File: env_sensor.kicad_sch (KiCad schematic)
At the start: 40 parts, among them J1 E Paper, J10 PWMOUT, J15 MH-Z19, J16 ADCs, J18 Conn_01x02_Pin, J3 Barrel_Jack, J4 LED_OUTPUT, J7 USB_C_Receptacle_USB2.0_16P, J8 v5_v3, J9 DEBUG, Q1 NMOS, Q2 NMOS, Q3 NMOS, SW1 EN, SW2 BOOT, U3 ESP32-S3-WROOM-1, U4 TXB0104PW, U6 TPS2065CDBV, U7 AP7361C-33E, Y1 Crystal

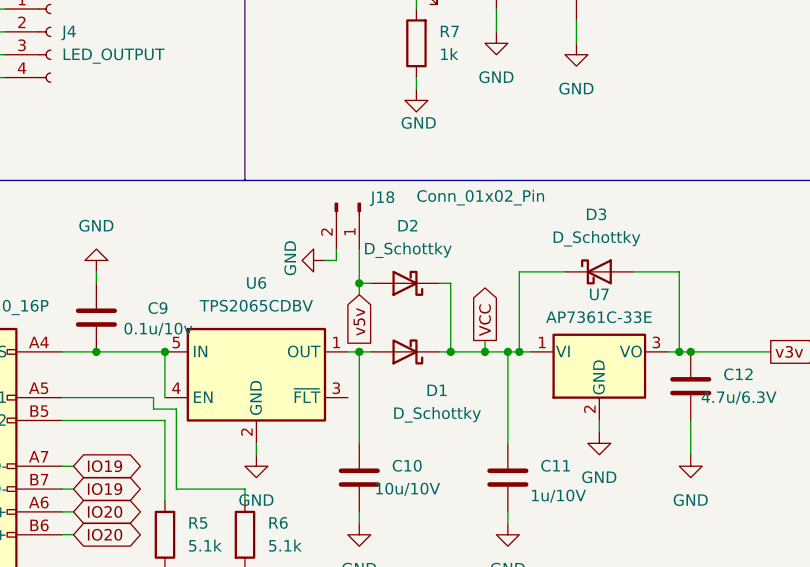
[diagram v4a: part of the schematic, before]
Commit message: update BOM
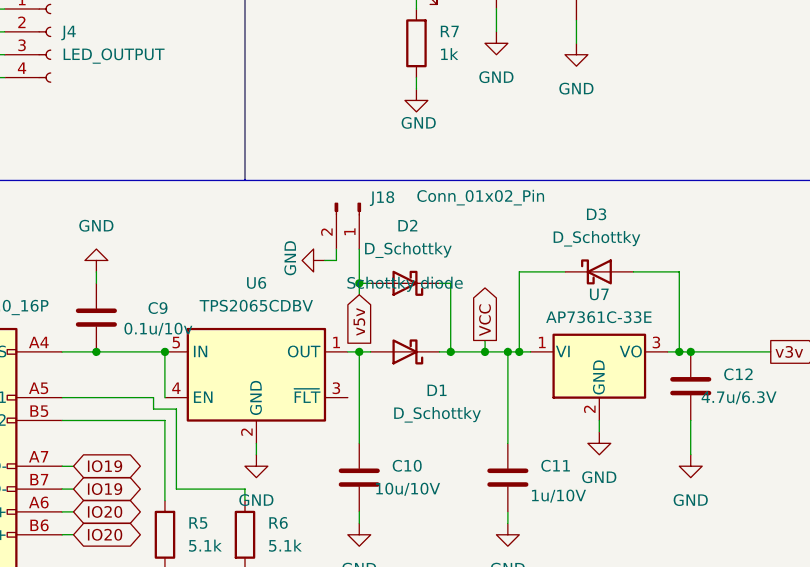
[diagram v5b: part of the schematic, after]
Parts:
- C7, C9: LCSC (none) -> C1853272
- D1, D2, D3: LCSC C86598 -> C123070
- R4: LCSC (none) -> C25804
- R5, R6: LCSC (none) -> C23186
- U6: LCSC (none) -> C353882
- U7: LCSC (none) -> C500795
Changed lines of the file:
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@@
 			)
 		)
-		(property "LCSC" ""
+		(property "LCSC" "C1853272"
 			(at 53.34 148.59 90)
 			(effects
@@
 			)
 		)
-		(property "LCSC" ""
+		(property "LCSC" "C25804"
 			(at 144.78 41.91 0)
 			(effects
@@
 			)
 		)
+		(property "LCSC" "C500795"
+			(at 109.22 152.4 0)
+			(effects
+				(font
+					(size 1.27 1.27)
+				)
+				(hide yes)
+			)
+		)
 		(pin "1"
 		)
@@
 			)
 		)
-		(property "LCSC" ""
+		(property "LCSC" "C23186"
 			(at 60.96 172.72 0)
 			(effects
@@
 			)
 		)
-		(property "LCSC" "C86598"
+		(property "LCSC" "C123070"
 			(at 109.22 143.51 0)
 			(effects
@@
 			)
 		)
-		(property "LCSC" ""
+		(property "LCSC" "C1853272"
 			(at 175.26 41.91 90)
 			(effects
@@
 			)
 		)
+		(property "LCSC" "C353882"
+			(at 71.12 154.94 0)
+			(effects
+				(font
+					(size 1.27 1.27)
+				)
+				(hide yes)
+			)
+		)
 		(pin "1"
 		)
@@
 			)
 		)
-		(property "LCSC" "C86598"
+		(property "LCSC" "C123070"
 			(at 87.63 152.4 0)
 			(effects
@@
 			)
 		)
-		(property "LCSC" ""
+		(property "LCSC" "C23186"
 			(at 69.85 172.72 0)
 			(effects
@@
 					(size 1.27 1.27)
 				)
-				(hide yes)
 			)
 		)
-		(property "LCSC" "C86598"
+		(property "LCSC" "C123070"
 			(at 87.63 144.78 0)
 			(effects

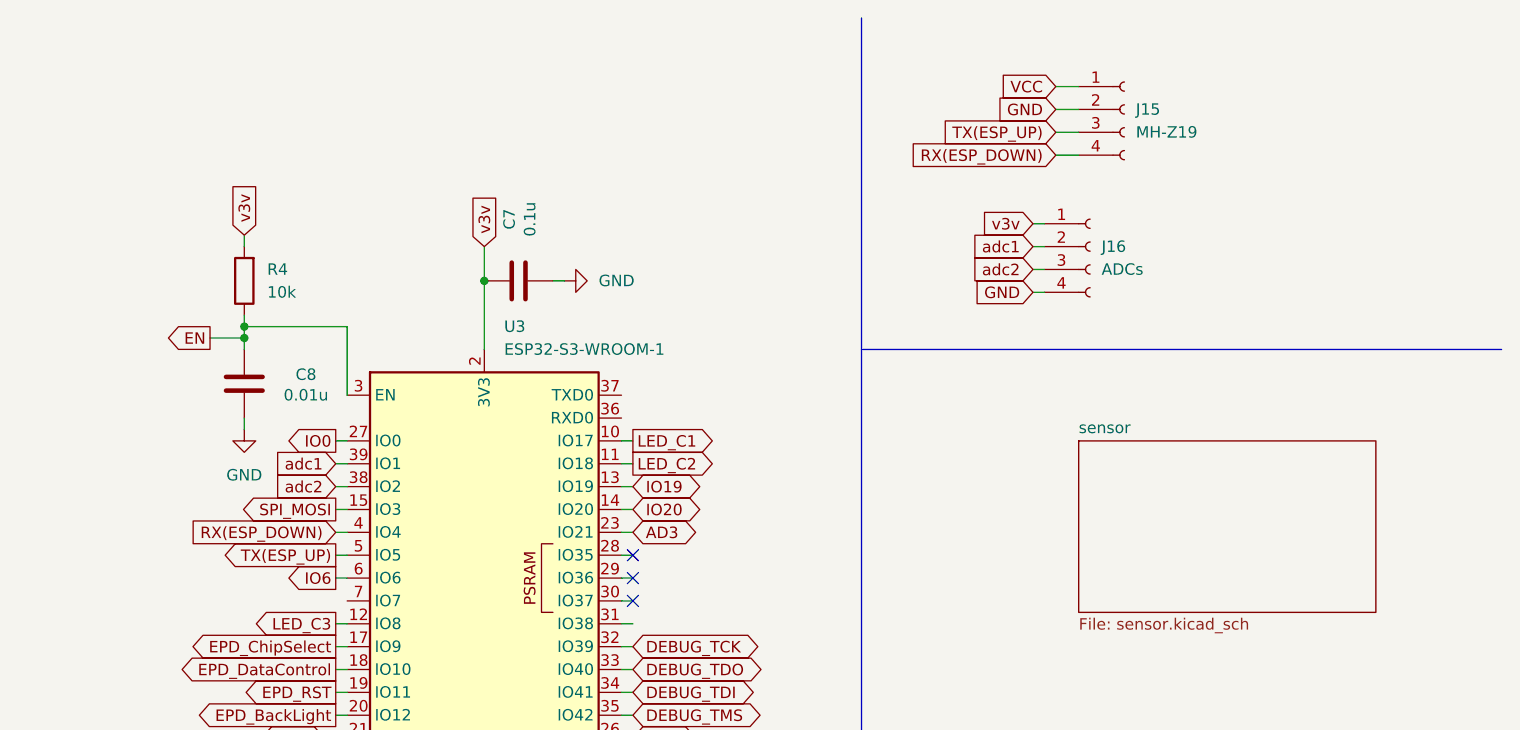
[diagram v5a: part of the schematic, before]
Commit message: ok
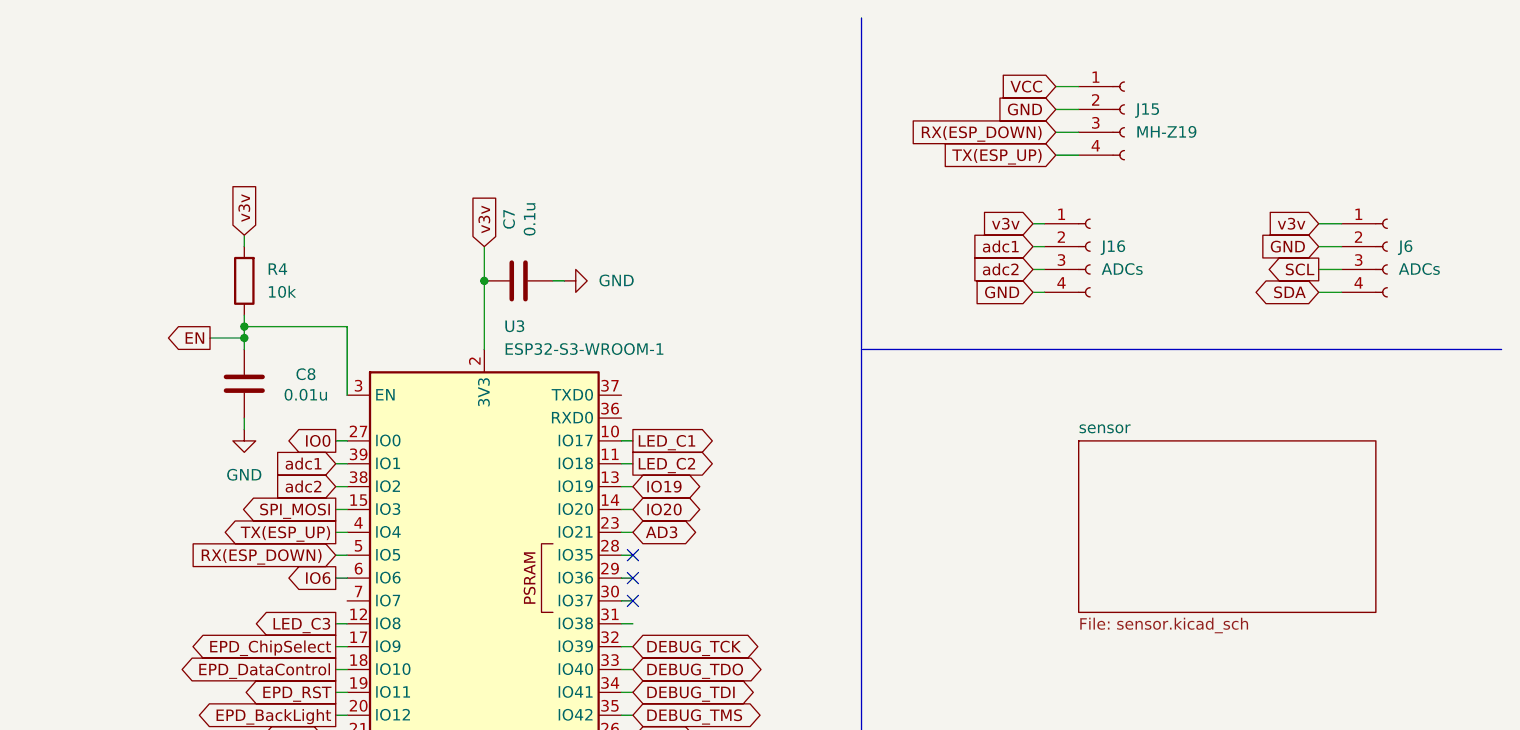
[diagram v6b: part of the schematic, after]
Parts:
- added J6: ADCs, Connector_PinSocket_2.54mm:PinSocket_1x04_P2.54mm_Vertical, symbol Connector:Conn_01x04_Socket
- C1, C4, C5: LCSC C14663 -> C1525
- C10, C6: LCSC C5137578 -> C19702
- C11: LCSC C5137578 -> C363553
- C12: LCSC C5137578 -> C380326
- C13, C14: LCSC (none) -> C5360831
- C7, C9: LCSC C1853272 -> C1525
- C8: LCSC (none) -> C307477
- J7: footprint Connector_USB:USB_C_Receptacle_GCT_USB4105-xx-A_16P_TopMnt_Horizontal -> Connector_USB:USB_C_Receptacle_GCT_USB4085; LCSC (none) -> C7095263
- Y1: LCSC (none) -> C1669858
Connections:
- net GND: now also J6.2 (Pin_2)
- net RX(ESP_DOWN): now also J15.3 (Pin_3), U3.5 (IO5); no longer J15.4 (Pin_4), U3.4 (IO4)
- net SCL: now also J6.3 (Pin_3)
- net SDA: now also J6.4 (Pin_4)
- net TX(ESP_UP): now also J15.4 (Pin_4), U3.4 (IO4); no longer J15.3 (Pin_3), U3.5 (IO5)
- net v3v: now also J6.1 (Pin_1)

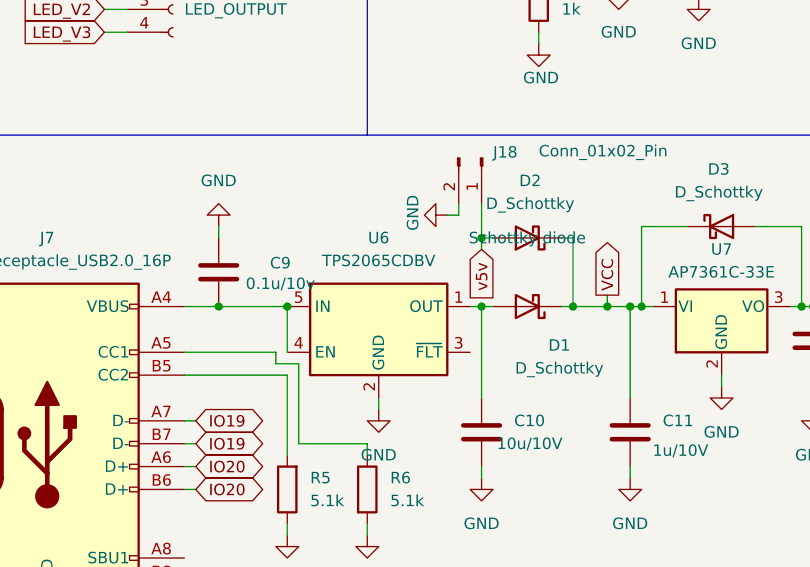
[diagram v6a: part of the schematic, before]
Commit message: update
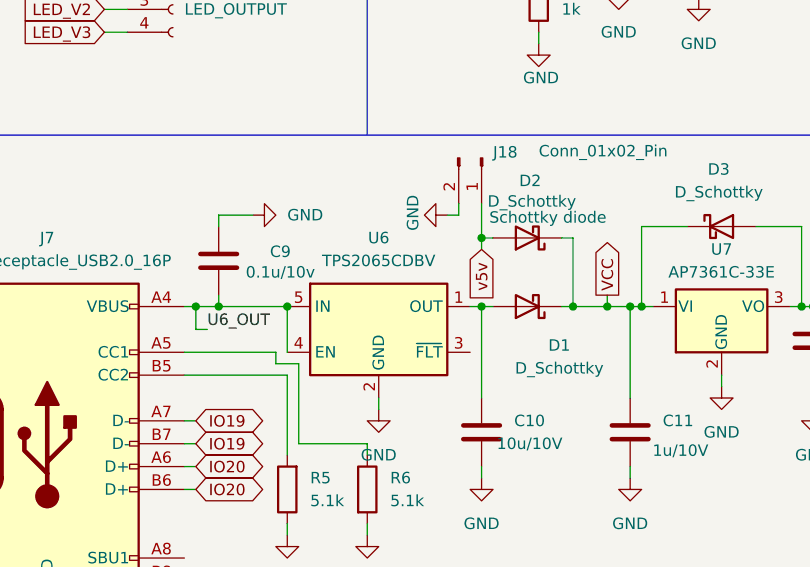
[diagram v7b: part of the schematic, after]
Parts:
- C8: LCSC C307477 -> C136131
- J10, J18, J9, U3: now left out of the parts list
- Q1, Q2: LCSC C916396 -> C557932
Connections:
- net U6_OUT: now reaches C9.2, J7.A4 (VBUS), J7.A9 (VBUS), J7.B4 (VBUS), J7.B9 (VBUS), U6.4 (EN), U6.5 (IN)
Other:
- moved on the sheet: C9
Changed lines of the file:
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@@
 	)
 	(junction
+		(at 50.8 152.4)
+		(diameter 0)
+		(color 0 0 0 0)
+	)
+	(junction
 		(at 171.45 41.91)
 		(diameter 0)
@@
 	(wire
 		(pts
-			(xy 82.55 162.56) (xy 82.55 152.4)
-		)
-		(stroke
-			(width 0)
-			(type default)
-		)
-	)
-	(wire
-		(pts
 			(xy 53.34 66.04) (xy 57.15 66.04)
 		)
@@
 	(wire
 		(pts
-			(xy 53.34 143.51) (xy 53.34 144.78)
-		)
-		(stroke
-			(width 0)
-			(type default)
-		)
-	)
-	(wire
-		(pts
 			(xy 40.64 114.3) (xy 43.18 114.3)
 		)
@@
 	(wire
 		(pts
-			(xy 53.34 152.4) (xy 49.53 152.4)
+			(xy 53.34 152.4) (xy 50.8 152.4)
 		)
 		(stroke
@@
 	(wire
 		(pts
+			(xy 82.55 152.4) (xy 82.55 162.56)
+		)
+		(stroke
+			(width 0)
+			(type default)
+		)
+	)
+	(wire
+		(pts
 			(xy 50.8 167.64) (xy 49.53 167.64)
 		)
@@
 	(wire
 		(pts
+			(xy 57.15 142.24) (xy 53.34 142.24)
+		)
+		(stroke
+			(width 0)
+			(type default)
+		)
+	)
+	(wire
+		(pts
 			(xy 186.69 92.71) (xy 187.96 92.71)
 		)
@@
 	(wire
 		(pts
+			(xy 53.34 142.24) (xy 53.34 143.51)
+		)
+		(stroke
+			(width 0)
+			(type default)
+		)
+	)
+	(wire
+		(pts
 			(xy 236.22 116.84) (xy 245.11 116.84)
 		)
@@
 	(wire
 		(pts
+			(xy 53.34 151.13) (xy 53.34 152.4)
+		)
+		(stroke
+			(width 0)
+			(type default)
+		)
+	)
+	(wire
+		(pts
 			(xy 236.22 134.62) (xy 236.22 133.35)
 		)
@@
 	(wire
 		(pts
+			(xy 50.8 154.94) (xy 50.8 152.4)
+		)
+		(stroke
+			(width 0)
+			(type default)
+		)
+	)
+	(wire
+		(pts
 			(xy 234.95 27.94) (xy 237.49 27.94)
 		)
@@
 		)
 	)
+	(wire
+		(pts
+			(xy 50.8 152.4) (xy 49.53 152.4)
+		)
+		(stroke
+			(width 0)
+			(type default)
+		)
+	)
 	(polyline
 		(pts
@@
 	(wire
 		(pts
+			(xy 52.07 154.94) (xy 50.8 154.94)
+		)
+		(stroke
+			(width 0)
+			(type default)
+		)
+	)
+	(wire
+		(pts
 			(xy 187.96 69.85) (xy 186.69 69.85)
 		)
@@
 		)
 	)
+	(label "U6_OUT"
+		(at 52.07 154.94 0)
+		(fields_autoplaced yes)
+		(effects
+			(font
+				(size 1.27 1.27)
+			)
+			(justify left bottom)
+		)
+	)
 	(label "VServo"
 		(at 250.19 114.3 0)
@@
 		(unit 1)
 		(exclude_from_sim no)
-		(in_bom yes)
+		(in_bom no)
 		(on_board yes)
 		(dnp no)
@@
 	(symbol
 		(lib_id "Device:C")
-		(at 53.34 148.59 0)
+		(at 53.34 147.32 0)
 		(unit 1)
 		(exclude_from_sim no)
@@
 		(dnp no)
 		(property "Reference" "C9"
-			(at 60.198 147.574 0)
+			(at 60.198 146.304 0)
 			(effects
 				(font
@@
 		)
 		(property "Value" "0.1u/10v"
-			(at 60.198 149.86 0)
+			(at 60.198 148.59 0)
 			(effects
 				(font
@@
 		)
 		(property "Footprint" "Capacitor_SMD:C_0603_1608Metric"
-			(at 54.3052 152.4 0)
+			(at 54.3052 151.13 0)
 			(effects
 				(font
@@
 		)
 		(property "Datasheet" "~"
-			(at 53.34 148.59 0)
+			(at 53.34 147.32 0)
 			(effects
 				(font
@@
 		)
 		(property "Description" ""
-			(at 53.34 148.59 0)
+			(at 53.34 147.32 0)
 			(effects
 				(font
@@
 		)
 		(property "LCSC" "C1525"
-			(at 53.34 148.59 90)
+			(at 53.34 147.32 90)
 			(effects
 				(font
@@
 		(unit 1)
 		(exclude_from_sim no)
-		(in_bom yes)
+		(in_bom no)
 		(on_board yes)
 		(dnp no)
@@
 		(exclude_from_sim no)
 		(in_bom no)
-		(on_board no)
+		(on_board yes)
 		(dnp no)
 		(fields_autoplaced yes)
@@
 	(symbol
 		(lib_id "power:GND")
-		(at 53.34 143.51 180)
+		(at 57.15 142.24 90)
 		(unit 1)
 		(exclude_from_sim no)
@@
 		(fields_autoplaced yes)
 		(property "Reference" "#PWR010"
-			(at 53.34 137.16 0)
+			(at 63.5 142.24 0)
 			(effects
 				(font
@@
 		)
 		(property "Value" "GND"
-			(at 53.34 138.43 0)
+			(at 60.96 142.2399 90)
 			(effects
 				(font
 					(size 1.27 1.27)
 				)
+				(justify right)
 			)
 		)
 		(property "Footprint" ""
-			(at 53.34 143.51 0)
+			(at 57.15 142.24 0)
 			(effects
 				(font
@@
 		)
 		(property "Datasheet" ""
-			(at 53.34 143.51 0)
+			(at 57.15 142.24 0)
 			(effects
 				(font
@@
 		)
 		(property "Description" "Power symbol creates a global label with name \"GND\" , ground"
-			(at 53.34 143.51 0)
+			(at 57.15 142.24 0)
 			(effects
 				(font
@@
 			)
 		)
-		(property "LCSC" "C916396"
+		(property "LCSC" "C557932"
 			(at 50.8 71.12 0)
 			(effects
@@
 			)
 		)
-		(property "LCSC" "C916396"
+		(property "LCSC" "C557932"
 			(at 50.8 45.72 0)
 			(effects
@@
 		(exclude_from_sim no)
 		(in_bom no)
-		(on_board no)
+		(on_board yes)
 		(dnp no)
 		(fields_autoplaced yes)
@@
 		(unit 1)
 		(exclude_from_sim no)
-		(in_bom yes)
+		(in_bom no)
 		(on_board yes)
 		(dnp no)
@@
 			)
 		)
-		(property "LCSC" "C307477"
+		(property "LCSC" "C136131"
 			(at 144.78 53.34 90)
 			(effects
@@
 		(unit 1)
 		(exclude_from_sim no)
-		(in_bom yes)
+		(in_bom no)
 		(on_board yes)
 		(dnp no)
@@
 		(on_board yes)
 		(dnp no)
-		(fields_autoplaced yes)
 		(property "Reference" "D2"
 			(at 87.9475 138.43 0)
@@
 		)
 		(property "Value" "D_Schottky"
-			(at 87.9475 140.97 0)
+			(at 88.138 140.716 0)
 			(effects
 				(font
@@
 		)
 		(property "Description" "Schottky diode"
-			(at 87.63 144.78 0)
+			(at 89.916 142.494 0)
 			(effects
 				(font
